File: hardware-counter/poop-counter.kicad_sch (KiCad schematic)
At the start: 40 parts, among them J1 USB_C_Receptacle_USB2.0, J2 RJ12, J3 Barrel_Jack, J4 Screw_Terminal_01x02, J5 Conn_01x03_Male, J6 Conn_01x02_Male, J7 Conn_01x03_Male, U0 ESP8266EX, U1 AMS1117-3.3, U2 CP2102N-A01-GQFN24, U3 MAX485E, U4 W25Q32JVSS, Y1 24Mhz±10ppm

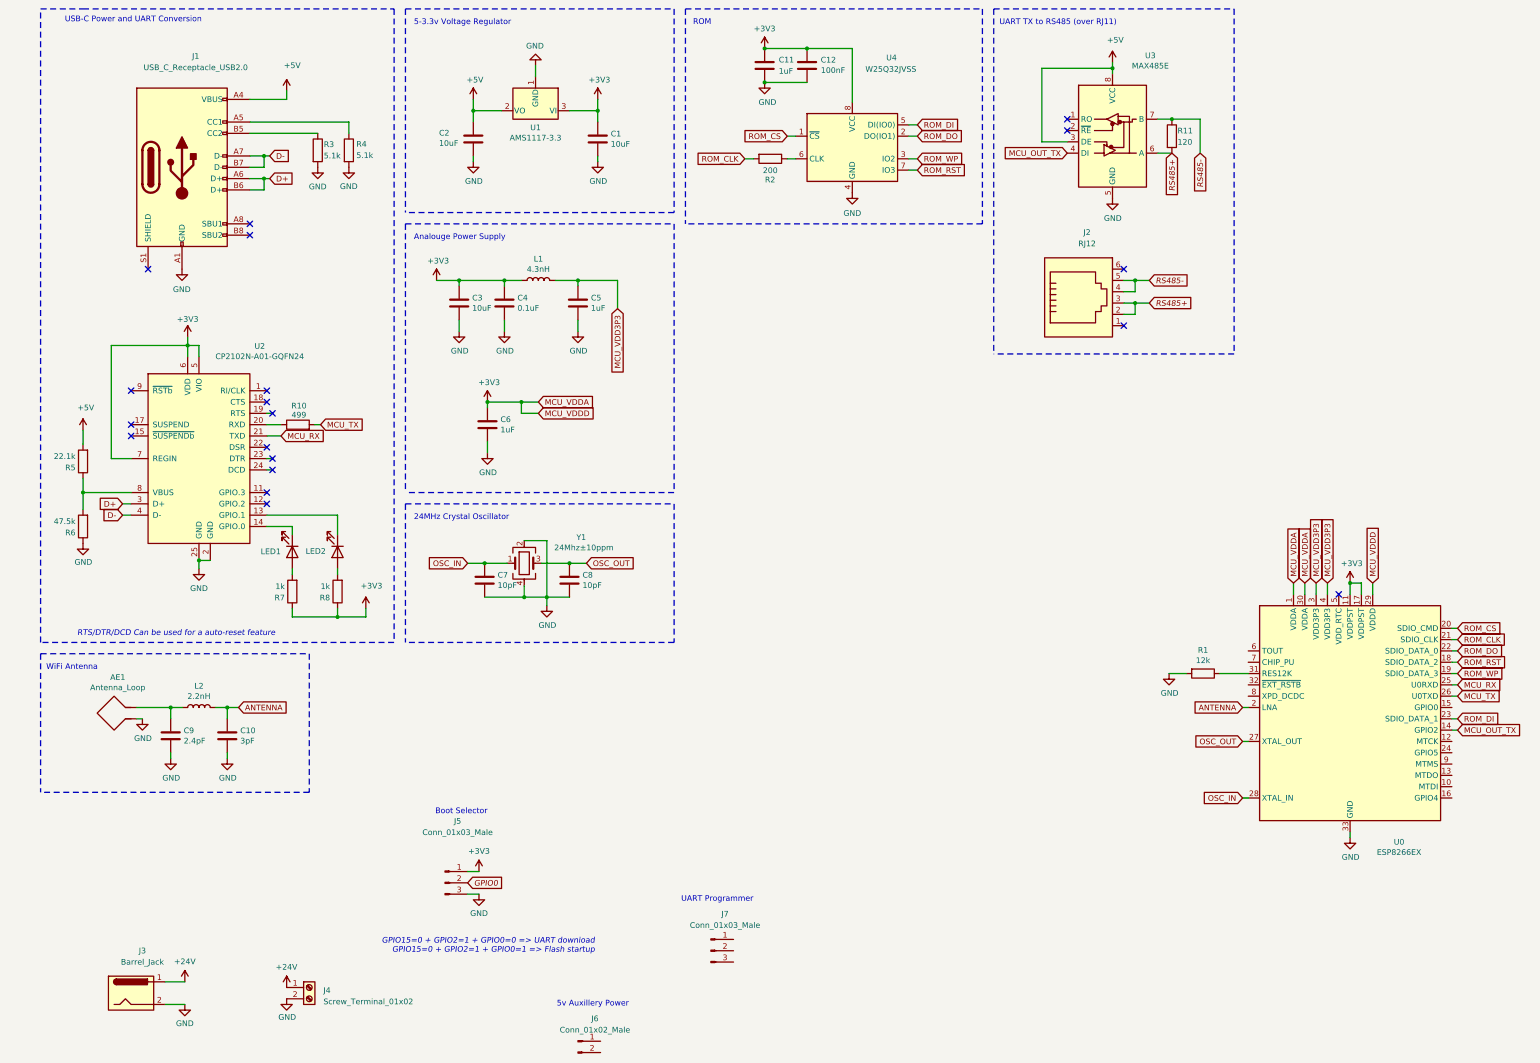
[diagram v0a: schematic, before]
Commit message: done v1, need to redo routing entirely lol
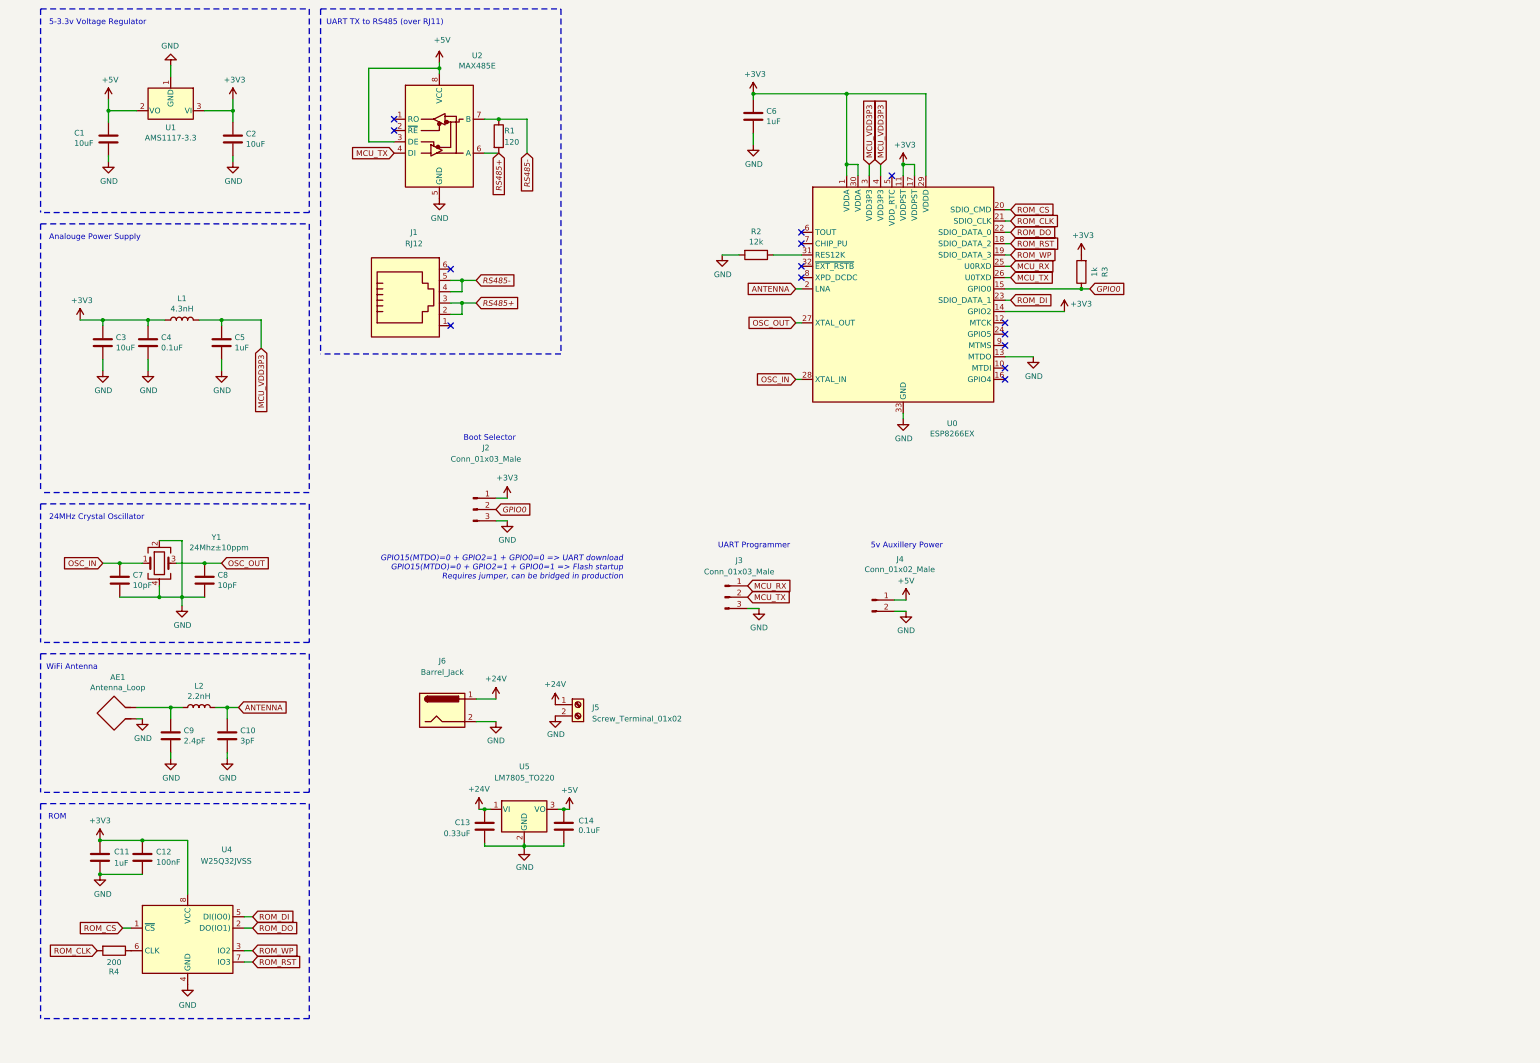
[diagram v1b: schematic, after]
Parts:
- removed D1: LED1, LED_SMD:LED_0805_2012Metric_Pad1.15x1.40mm_HandSolder, symbol Device:LED
- removed D2: LED2, LED_SMD:LED_0805_2012Metric_Pad1.15x1.40mm_HandSolder, symbol Device:LED
- removed J1: USB_C_Receptacle_USB2.0, Connector_USB:USB_C_Receptacle_Palconn_UTC16-G, symbol Connector:USB_C_Receptacle_USB2.0
- removed R10: 499, Resistor_SMD:R_0805_2012Metric_Pad1.20x1.40mm_HandSolder, symbol Device:R
- removed R4: 5.1k, Resistor_SMD:R_0805_2012Metric_Pad1.20x1.40mm_HandSolder, symbol Device:R
- removed R5: 22.1k, Resistor_SMD:R_0805_2012Metric_Pad1.20x1.40mm_HandSolder, symbol Device:R
- removed R6: 47.5k, Resistor_SMD:R_0805_2012Metric_Pad1.20x1.40mm_HandSolder, symbol Device:R
- removed R7, R8: 1k, Resistor_SMD:R_0805_2012Metric_Pad1.20x1.40mm_HandSolder, symbol Device:R
- removed U2: CP2102N-A01-GQFN24, Package_DFN_QFN:QFN-24-1EP_4x4mm_P0.5mm_EP2.6x2.6mm, symbol poop-counter-rescue:CP2102N-A01-GQFN24-Interface_USB
- added C13: 0.33uF, Capacitor_SMD:C_0805_2012Metric_Pad1.18x1.45mm_HandSolder, symbol Device:C
- added C14: 0.1uF, Capacitor_SMD:C_0805_2012Metric_Pad1.18x1.45mm_HandSolder, symbol Device:C
- added U5: LM7805_TO220, Package_TO_SOT_THT:TO-220-3_Vertical, symbol Regulator_Linear:LM7805_TO220
- R3: value 5.1k -> 1k
- Y1: footprint Crystal:Crystal_SMD_3225-4Pin_3.2x2.5mm_HandSoldering -> Crystal:Crystal_SMD_EuroQuartz_X22-4Pin_2.5x2.0mm
- renumbered C2 to C1, C1 to C2, J2 to J1, J5 to J2, J7 to J3, J6 to J4, J4 to J5, J3 to J6, R11 to R1, R1 to R2, R2 to R4, U3 to U2
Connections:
- net +24V: now also C13.2, U5.1 (VI)
- net +3V3: now also R3.2, U0.14 (GPIO2)
- net +5V: now also J4.1 (Pin_1), C14.1, U5.3 (VO)
- net GND: now also J3.3 (Pin_3), J4.2 (Pin_2), U0.13 (MTDO), C13.1, C14.2, U5.2 (GND); no longer R3.2
- net GPIO0: now also R3.1, U0.15 (GPIO0)
- net MCU_RX: now also J3.1 (Pin_1)
- net MCU_TX: now also J3.2 (Pin_2), U2.4 (DI)
- removed net MCU_OUT_TX: U0.14 (GPIO2), U2.4 (DI)
- no-connect marks 19 -> 14
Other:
- note added: "GPIO15(MTDO)=0 + GPIO2=1 + GPIO0=0 => UART download GPIO15(MTDO)=0 + GPIO2=1 + GPIO0=1 => Flash startup Requires jumper, can be bridged in production"
- note removed: "GPIO15=0 + GPIO2=1 + GPIO0=0 => UART download GPIO15=0 + GPIO2=1 + GPIO0=1 => Flash startup"
- note removed: "RTS/DTR/DCD Can be used for a auto-reset feature"
- note removed: "USB-C Power and UART Conversion"
- moved on the sheet: C1, C11, C12, C2, C3, C4, C5, C6, C7, C8, J1, J2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
